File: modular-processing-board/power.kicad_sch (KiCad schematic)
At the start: 10 parts, among them J301 Conn_02x06_Odd_Even, J701 Conn_02x02_Odd_Even, J702 Conn_02x03_Odd_Even, U701 AMS1117-3.3

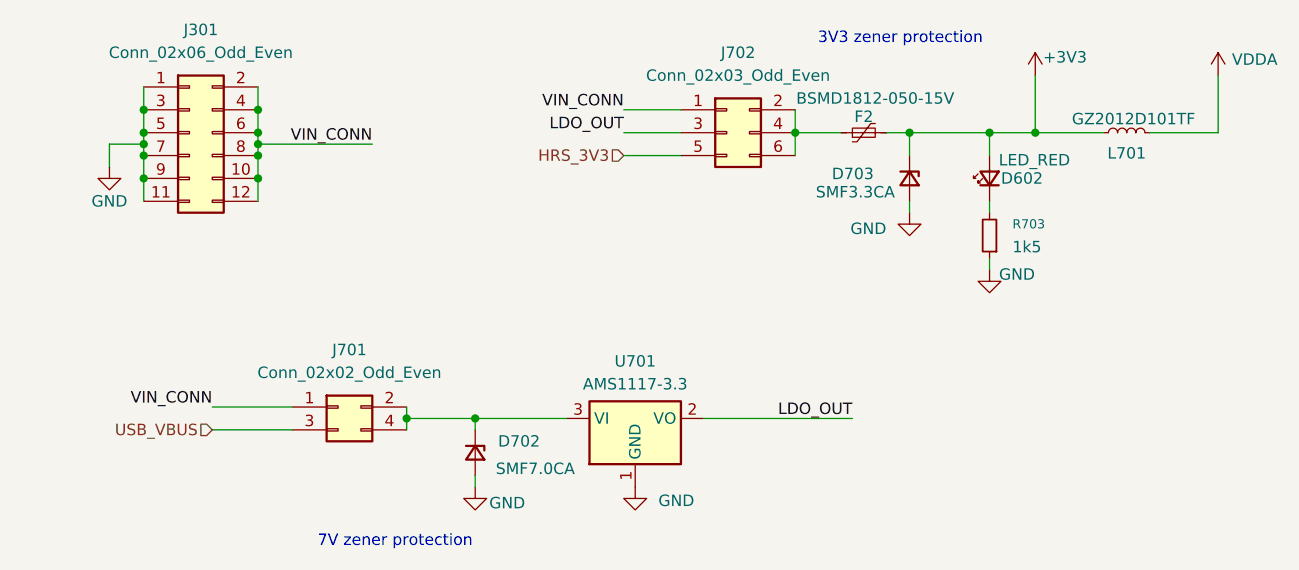
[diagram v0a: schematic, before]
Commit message: completed schematic
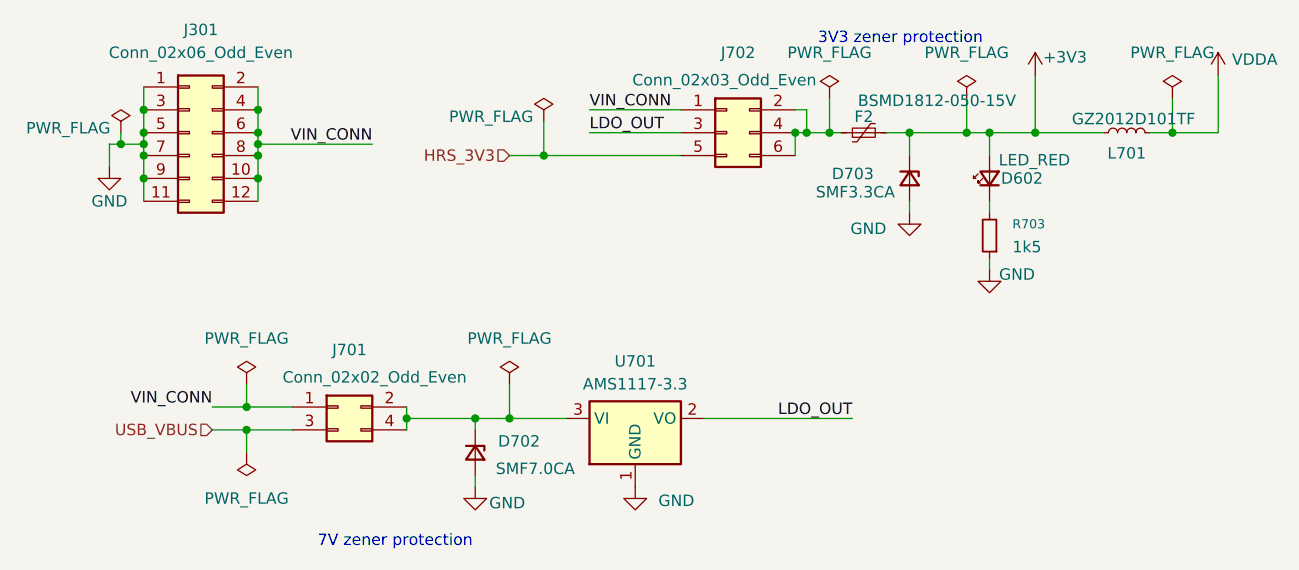
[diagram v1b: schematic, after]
